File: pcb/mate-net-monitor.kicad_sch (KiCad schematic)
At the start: 66 parts, among them J1 6P6C, J2 6P6C, J3 Conn_02x02_Odd_Even, J4 Conn_01x08, J5 RJHSE-5081, Q1 Si2337DS, U1 LM5085MY, U2 TLP185, U3 TLP185, U4 TLP185, U5 MAX3485

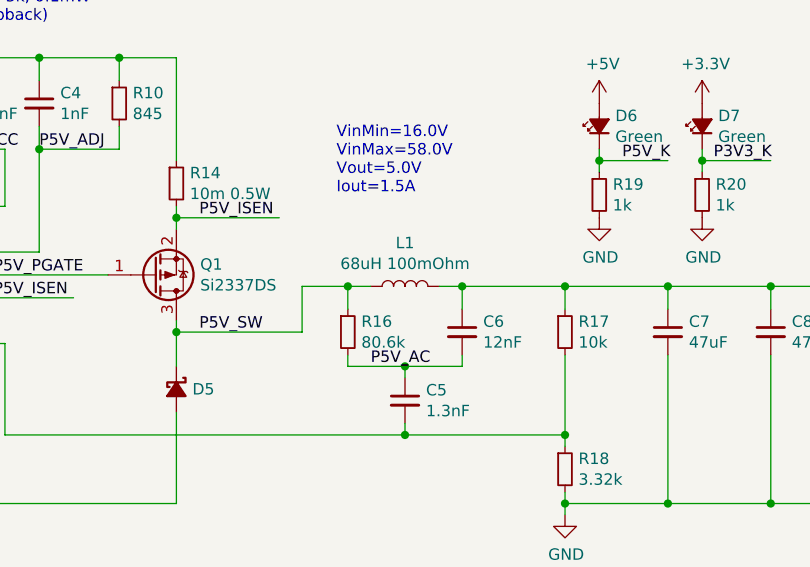
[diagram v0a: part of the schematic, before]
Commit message: sch notes and cleanup
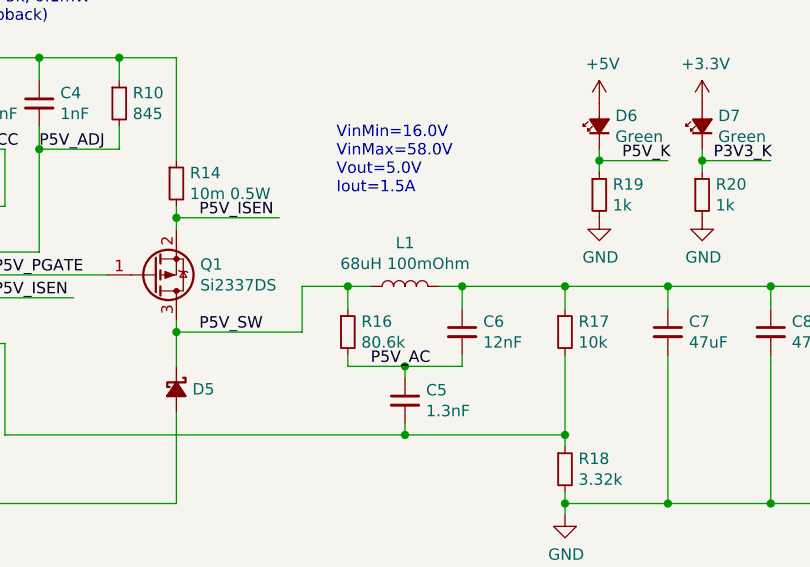
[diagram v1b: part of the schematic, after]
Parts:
- C1, C2: Mfg (none) -> TDK; Mfg PN (none) -> C3225X7S2A335K200AB
